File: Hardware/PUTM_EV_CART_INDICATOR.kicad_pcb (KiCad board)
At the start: 2 copper layers, 43 x 25 mm, 17 parts, among them J1 Screw_Terminal_01x08, K3 IM07DTS, K4 IM07DTS

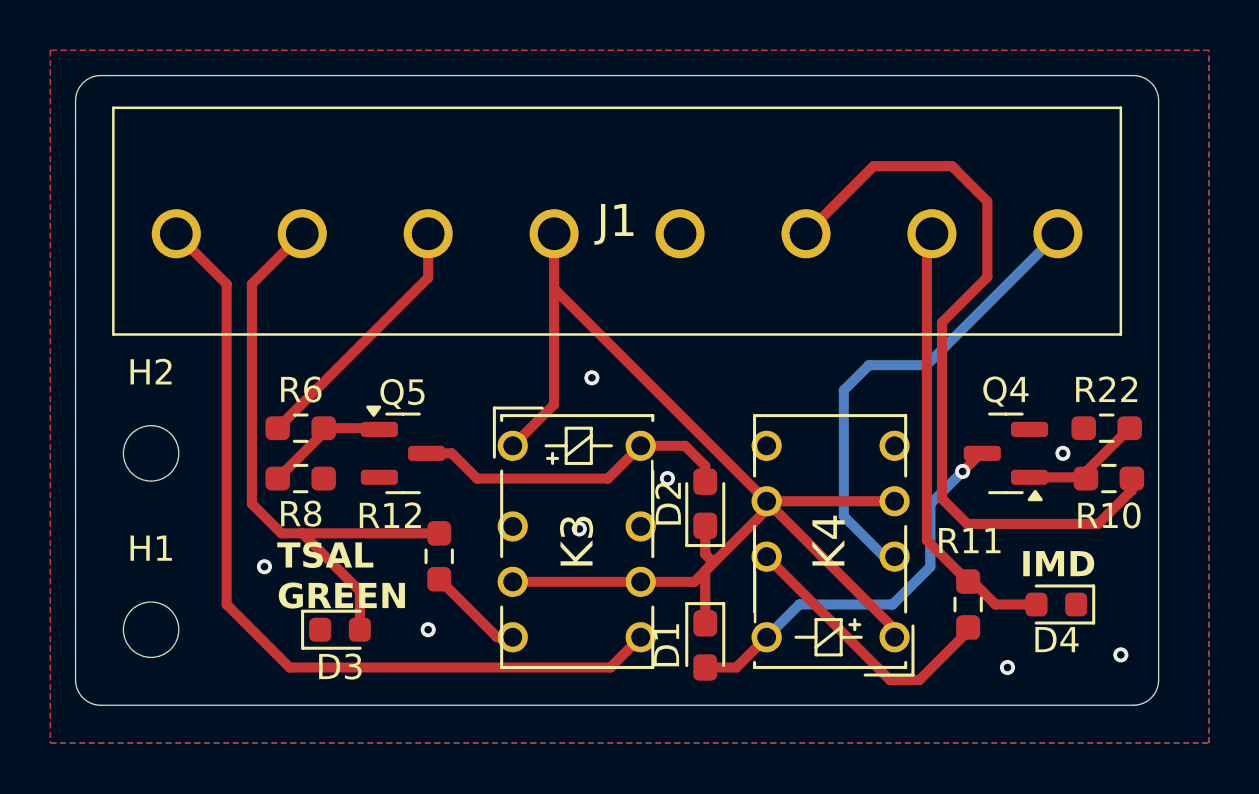
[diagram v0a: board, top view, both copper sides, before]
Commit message: poprawy diod
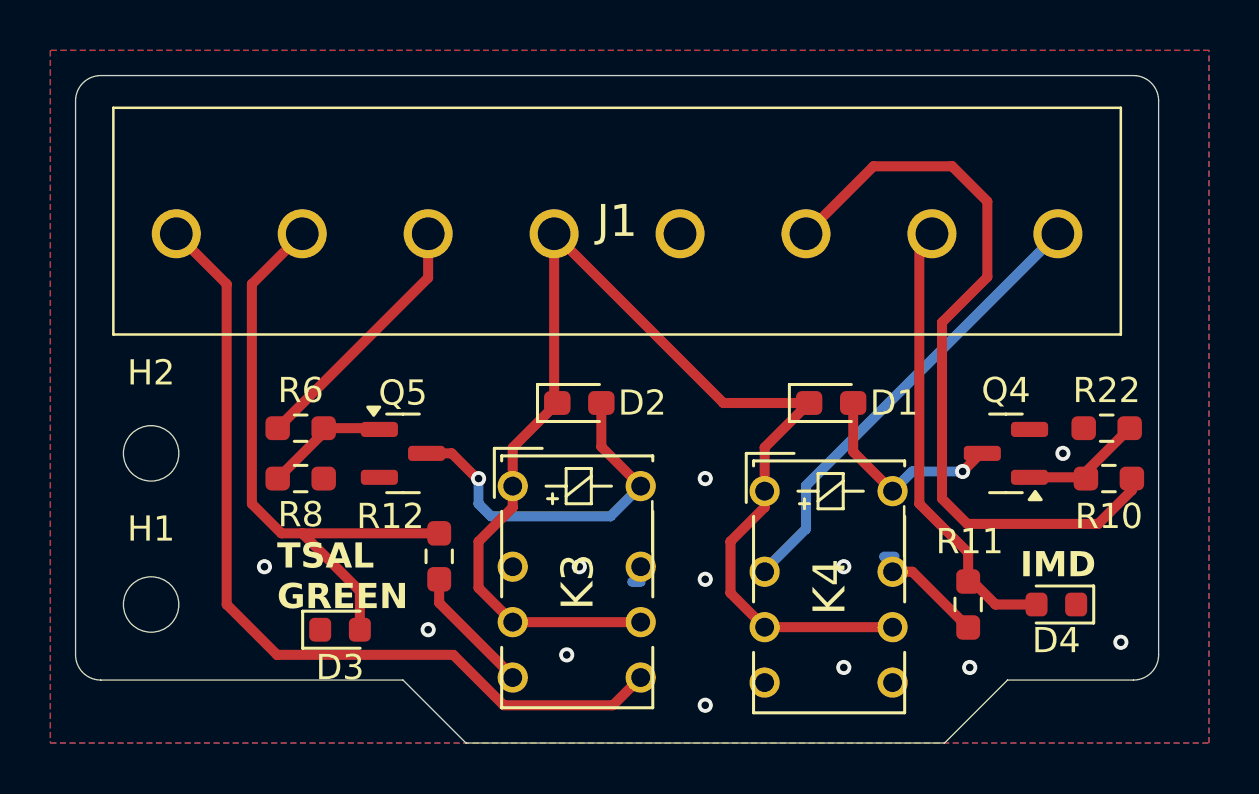
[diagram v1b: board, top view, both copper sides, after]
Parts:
- moved D1 10.8 mm to (112.0, 72.0), turned to 0 degrees
- moved D2 6.40 mm to (102.0, 72.0), turned to 0 degrees
- moved K4 1.80 mm to (111.9, 79.3), turned to -90 degrees
- moved K3 1.60 mm to (101.9, 79.1)
- moved H1 1.00 mm to (85.0, 80.0)
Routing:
- net Net-(D1-A): track 16.0 -> 8.33 mm
- net Net-(K4-NC_2): track 11.0 -> 4.48 mm
- net +24V: track 49.4 -> 51.5 mm
- net Net-(D2-A): track 13.0 -> 14.6 mm, vias 0 -> 1
- net Net-(K3-NO_1): track 3.87 -> 5.11 mm
- net /TSAL_COLUMN: track 33.5 -> 34.1 mm
- net /IMD_COLUMN: track 18.8 -> 18.2 mm
- net GND: vias 8 -> 12
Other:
- board size 43 x 25 mm -> 43 x 26.5 mm
